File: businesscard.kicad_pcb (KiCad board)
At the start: 2 copper layers, 88.9 x 50.8 mm, 12 parts, among them J1 Conn_01x08_Pin

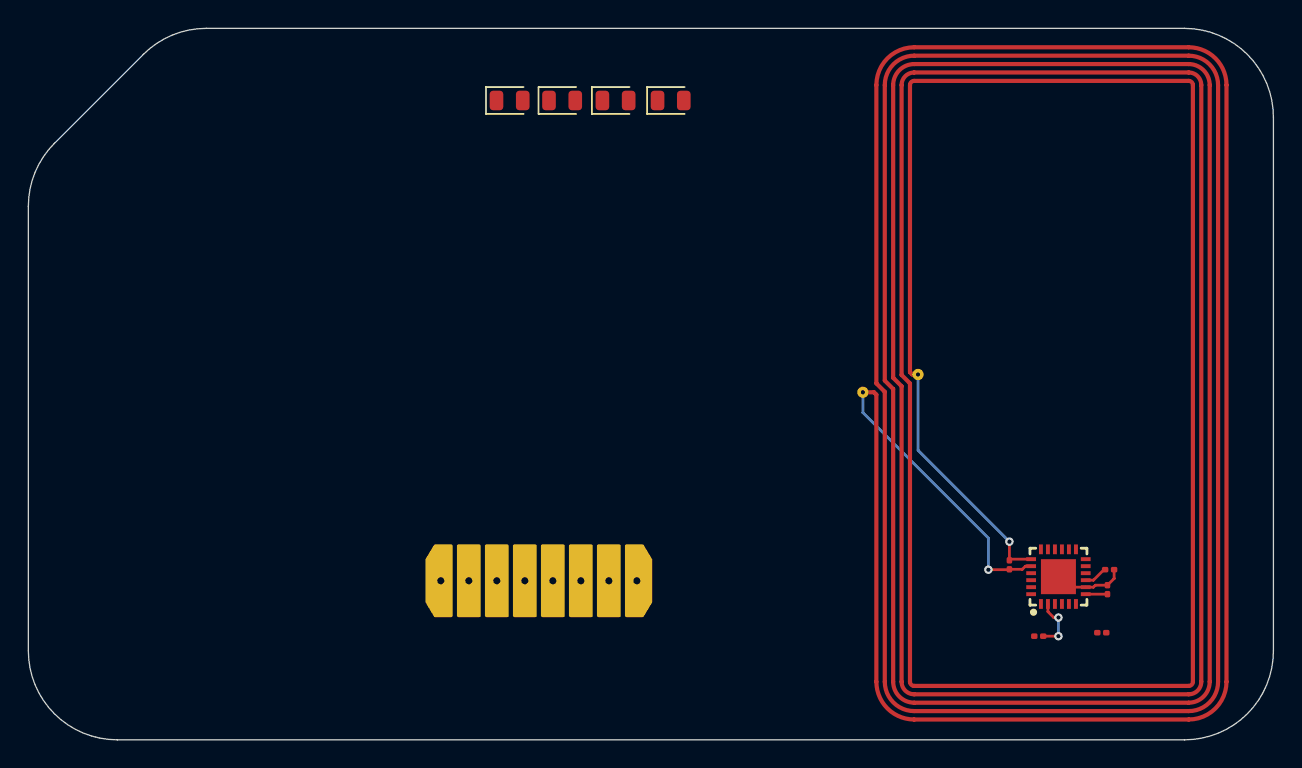
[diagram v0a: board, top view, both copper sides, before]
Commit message: finish pcb routing
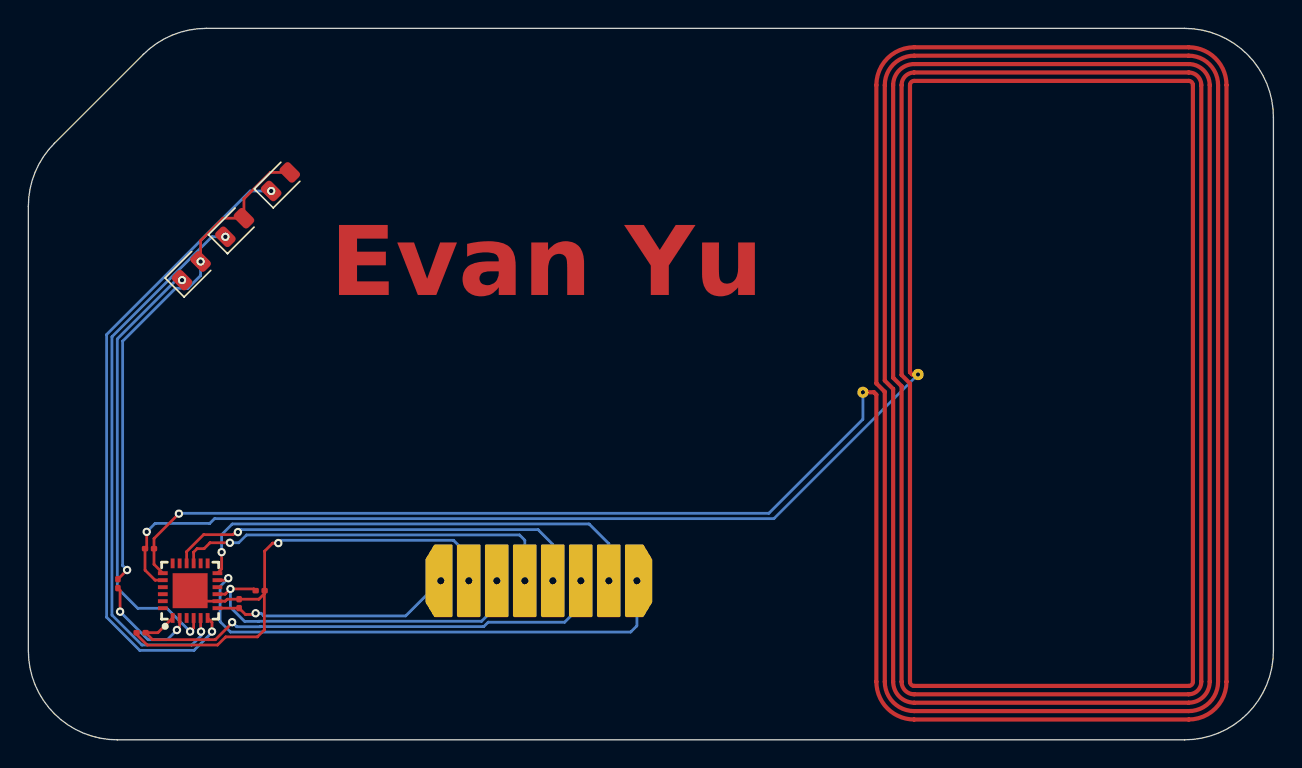
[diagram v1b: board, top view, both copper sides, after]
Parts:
- removed D4: LED, LED_SMD:LED_0805_2012Metric
- added REF**: HoldingHole, Library:HoldingHole, F.Cu at (124.5, 73.5)
- added REF**: Name_1, Library:Name_1, F.Cu at (129.5, 89.5)
- moved C4 68.6 mm to (116.0, 113.0), turned to 180 degrees
- moved R1 65.9 mm to (114.3, 109.5), turned to 90 degrees
- moved C2 62.0 mm to (123.0, 110.9)
- moved U2 62.0 mm to (119.5, 110.0)
- moved C1 61.4 mm to (116.6, 107.0), turned to 0 degrees
- moved C3 60.7 mm to (124.5, 110.0)
- moved D1 25.8 mm to (119.6, 87.2), turned to 45 degrees
- moved D2 25.1 mm to (122.7, 84.1), turned to 45 degrees
- moved D3 24.6 mm to (126.0, 80.8), turned to 45 degrees
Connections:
- C4 pad 1: Net-(U2-PIO0_0/WAKEUP) -> /WAKE
- J1 pad 3: /SWDIO -> /RESET
- J1 pad 5: /RESET -> /SWDIO
- J1 pad 6: VCC -> /WAKE
- U2 pad 1: Net-(U2-PIO0_0/WAKEUP) -> /WAKE
- U2 pad 13: /LEDC4 -> unconnected-(U2-PIO0_7/CT16B_M1-Pad13)
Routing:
- net /LEDC3: track 0.00 -> 46.4 mm, vias 0 -> 2
- net Net-(U2-LA): track 19.5 -> 64.1 mm
- net Net-(U2-LB): track 17.6 -> 58.8 mm
- net /LEDC2: track 0.00 -> 39.7 mm, vias 0 -> 2
- net /SCL: track 0.00 -> 37.6 mm, vias 0 -> 1
- net /WAKE: track 0.00 -> 36.7 mm, vias 0 -> 1
- net Net-(D1-A): track 0.00 -> 36.6 mm, vias 0 -> 2
- net /SDA: track 0.00 -> 34.1 mm, vias 0 -> 1
- net GND: track 5.21 -> 38.9 mm, vias 0 -> 1
- net /LEDC1: track 0.00 -> 31.7 mm, vias 0 -> 2
- net /SWDIO: track 0.00 -> 30.7 mm, vias 0 -> 1
- net /SWCLK: track 0.00 -> 28.0 mm, vias 0 -> 1
- net /RESET: track 1.70 -> 25.9 mm, vias 0 -> 1
- net VCC: track 1.55 -> 17.3 mm, vias 0 -> 1
- net /LEDR1: track 3.89 -> 7.86 mm
